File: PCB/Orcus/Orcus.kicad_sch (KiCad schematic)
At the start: 78 parts, among them SW1 MX_LED, SW10 MX_LED, SW11 MX_LED, SW12 MX_LED, SW13 MX_LED, SW14 MX_LED, SW15 MX_LED, SW16 MX_LED, SW17 MX_LED, SW18 MX_LED, SW19 MX_LED, SW2 MX_LED, SW20 MX_LED, SW21 MX_LED, SW22 MX_LED, SW23 MX_LED, SW24 MX_LED, SW25 MX_LED, SW26 MX_LED, SW27 MX_LED, SW28 MX_LED, SW29 MX_LED, SW3 MX_LED, SW30 MX_LED, SW31 MX_LED, SW32 MX_LED, SW33 MX_LED, SW34 MX_LED, SW35 MX_LED, SW36 MX_LED, SW37 MX_LED, SW38 MX_LED, SW4 MX_LED, SW5 MX_LED, SW6 MX_LED, SW7 MX_LED, SW8 MX_LED, SW9 MX_LED, U1 SeeeduinoXIAO, U2 SeeeduinoXIAO

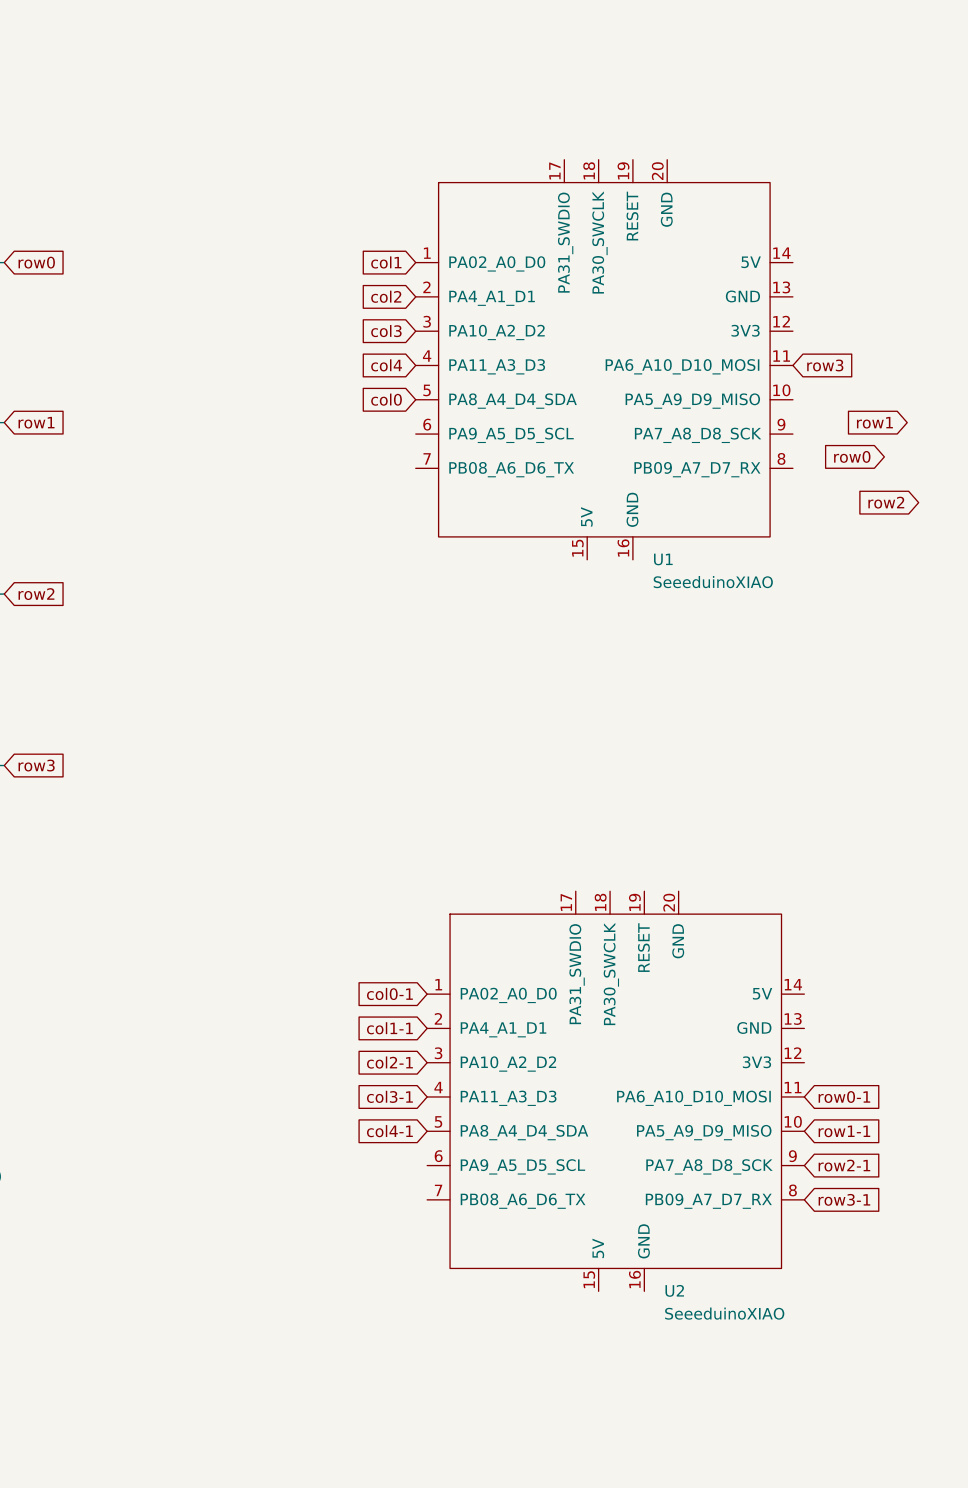
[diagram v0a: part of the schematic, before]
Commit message: traces remaining
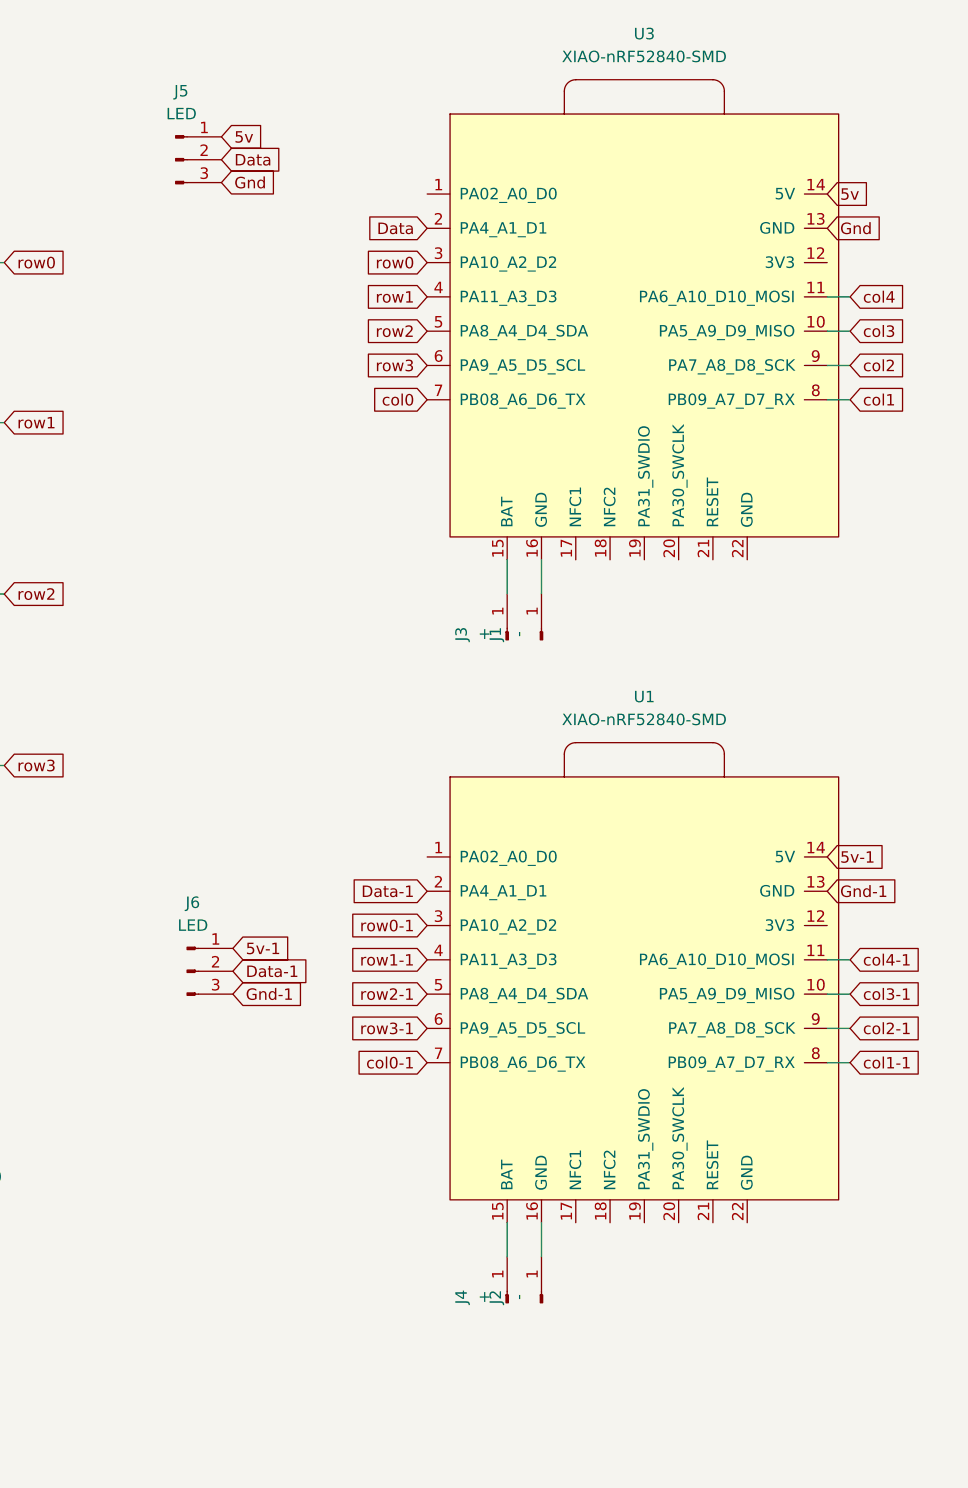
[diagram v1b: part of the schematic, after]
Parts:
- removed U1, U2: SeeeduinoXIAO, Seeeduino XIAO KICAD:Seeeduino XIAO-MOUDLE14P-2.54-21X17.8MM-holes, symbol Seeeduino XIAO:SeeeduinoXIAO
- added J1, J2: -, TOTEMlib:BatteryPad, symbol Connector:Conn_01x01_Pin
- added J3, J4: +, TOTEMlib:BatteryPad, symbol Connector:Conn_01x01_Pin
- added J5, J6: LED, Keebio-Parts.pretty-master:NeoPixel_Mini_Button-v2, symbol Connector:Conn_01x03_Pin
- added U1, U3: XIAO-nRF52840-SMD, TOTEMlib:xiao-ble-smd-cutout-mod, symbol MCU_SEEED_XIAO_Series:XIAO-nRF52840-SMD
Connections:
- net col0: now also U3.7 (PB08_A6_D6_TX)
- net col0-1: now also U1.7 (PB08_A6_D6_TX)
- net col1: now also U3.8 (PB09_A7_D7_RX)
- net col1-1: now also U1.8 (PB09_A7_D7_RX)
- net col2: now also U3.9 (PA7_A8_D8_SCK)
- net col2-1: now also U1.9 (PA7_A8_D8_SCK)
- net col3: now also U3.10 (PA5_A9_D9_MISO)
- net col3-1: now also U1.10 (PA5_A9_D9_MISO)
- net col4: now also U3.11 (PA6_A10_D10_MOSI)
- net col4-1: now also U1.11 (PA6_A10_D10_MOSI)
- net row0: now also U3.3 (PA10_A2_D2)
- net row0-1: now also U1.3 (PA10_A2_D2)
- net row1: now also U3.4 (PA11_A3_D3)
- net row1-1: now also U1.4 (PA11_A3_D3)
- net row2: now also U3.5 (PA8_A4_D4_SDA)
- net row2-1: now also U1.5 (PA8_A4_D4_SDA)
- net row3: now also U3.6 (PA9_A5_D5_SCL)
- net row3-1: now also U1.6 (PA9_A5_D5_SCL)
- new net: J4.1 (Pin_1), U1.15 (BAT)
- new net: J2.1 (Pin_1), U1.16 (GND)
- new net: J1.1 (Pin_1), U3.16 (GND)
- new net: J3.1 (Pin_1), U3.15 (BAT)
- new net 5v: J5.1 (Pin_1), U3.14 (5V)
- new net 5v-1: J6.1 (Pin_1), U1.14 (5V)
- new net Data: J5.2 (Pin_2), U3.2 (PA4_A1_D1)
- new net Data-1: J6.2 (Pin_2), U1.2 (PA4_A1_D1)
- new net Gnd: J5.3 (Pin_3), U3.13 (GND)
- new net Gnd-1: J6.3 (Pin_3), U1.13 (GND)
